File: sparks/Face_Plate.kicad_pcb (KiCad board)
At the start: 2 copper layers, 84 x 84 mm, 0 parts

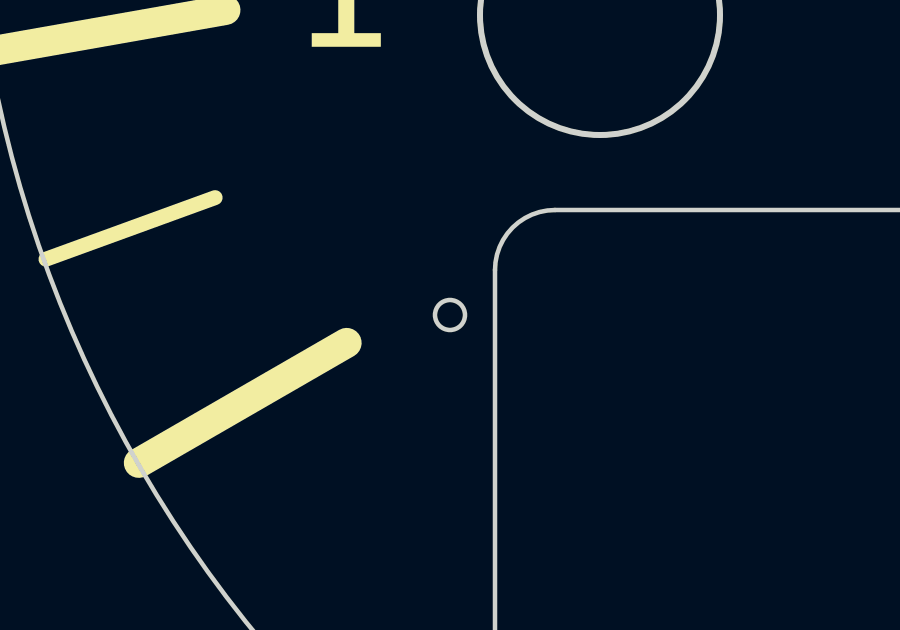
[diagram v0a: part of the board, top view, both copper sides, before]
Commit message: Stuff
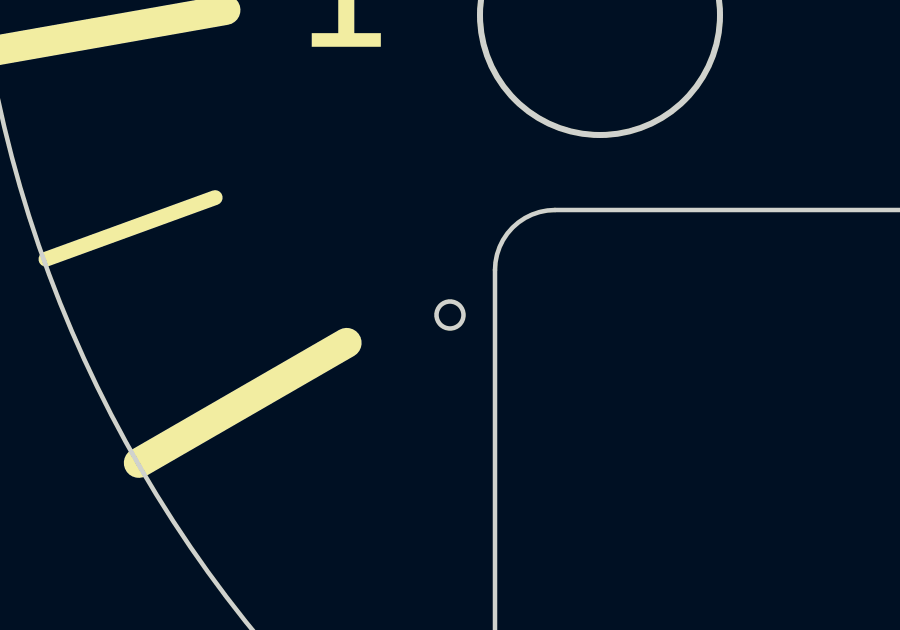
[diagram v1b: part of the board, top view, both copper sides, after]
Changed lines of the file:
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@@
     (uvia_drill 0.1)
   )
-  (gr_circle (center 124 116) (end 124.5 116) (layer Edge.Cuts) (width 0.15))
+  (gr_circle (center 124 116) (end 124.45 116) (layer Edge.Cuts) (width 0.15))
   (gr_circle (center 171 94) (end 175 94) (layer Edge.Cuts) (width 0.2))
   (gr_circle (center 171 106) (end 175 106) (layer Edge.Cuts) (width 0.2))
